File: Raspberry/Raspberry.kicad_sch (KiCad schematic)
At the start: 9 parts, among them J1 Conn_01x02_Pin, J2 Conn_01x04, J3 Conn_01x02_Pin, J4 Conn_01x06_Pin

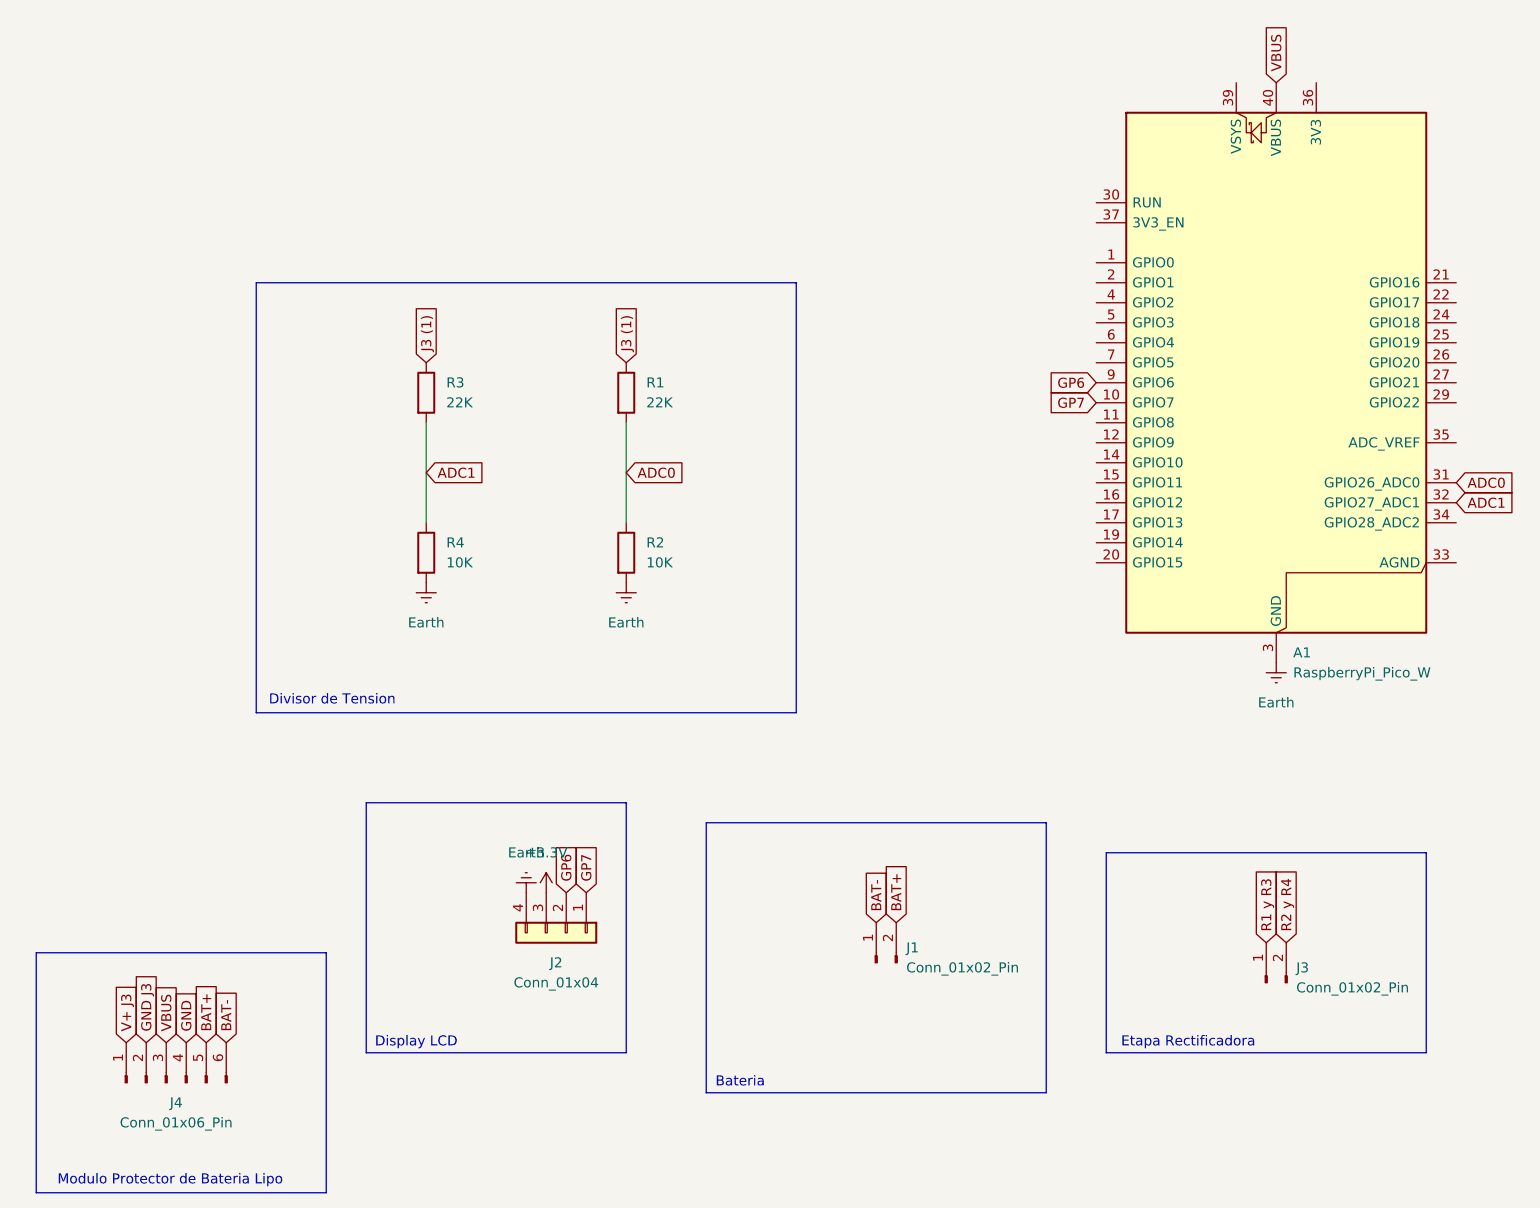
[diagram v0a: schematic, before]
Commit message: Actualización de la PCB, carpeta de campo
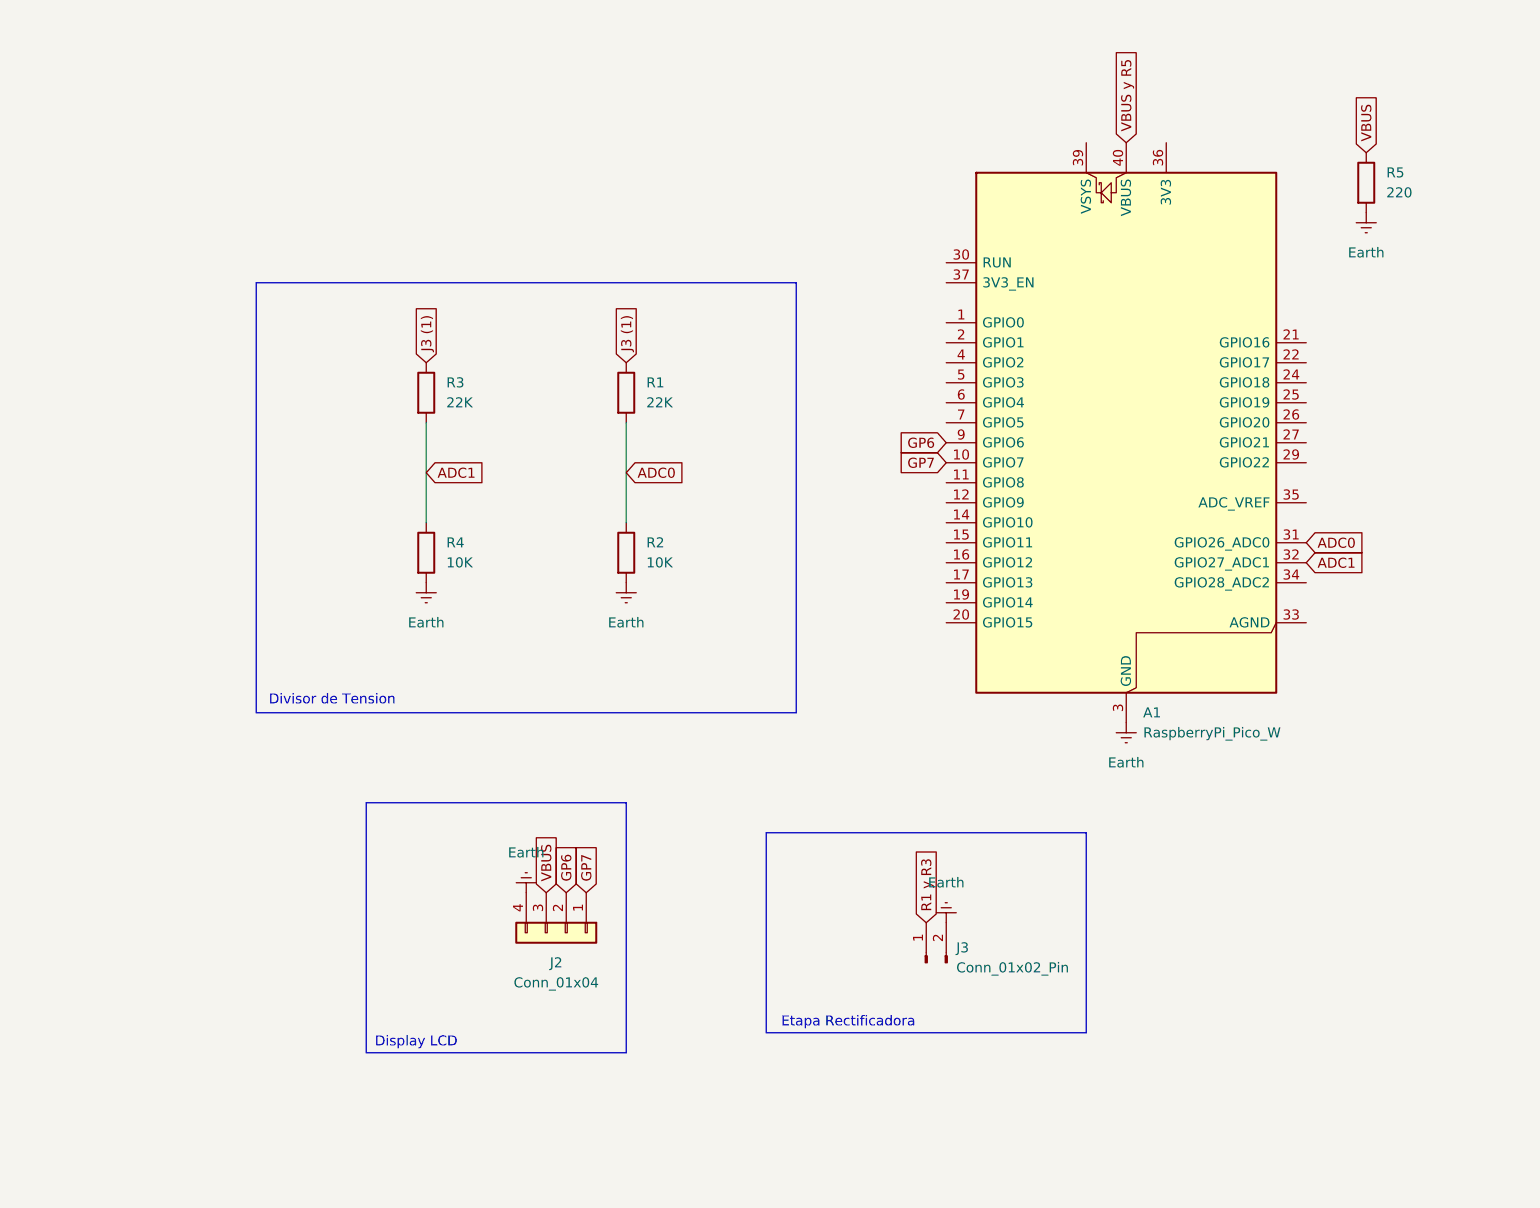
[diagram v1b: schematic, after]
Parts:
- removed J1: Conn_01x02_Pin, Connector_JST:JST_PH_B2B-PH-K_1x02_P2.00mm_Vertical, symbol Connector:Conn_01x02_Pin
- removed J4: Conn_01x06_Pin, Aura_de_modulo:TP4056-Module, symbol Connector:Conn_01x06_Pin
- added R5: 220, Resistor_THT:R_Axial_DIN0207_L6.3mm_D2.5mm_P2.54mm_Vertical, symbol Device:R
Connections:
- net +3.3V is gone; now on net VBUS: J2.3 (Pin_3)
- net R2 y R4 is gone; now on net Earth: J3.2 (Pin_2)
- net Earth: now also R5.2
- net VBUS: now also R5.1; no longer A1.40 (VBUS)
- new net VBUS y R5: A1.40 (VBUS)
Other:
- note removed: "Bateria"
- note removed: "Modulo Protector de Bateria Lipo"
- moved on the sheet: A1, J3
